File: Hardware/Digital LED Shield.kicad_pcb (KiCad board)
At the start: 2 copper layers, 22 x 26.5 mm, 17 parts, among them IC1 TPS2420RSAT, IC2 LM66200DRLR, J1 Conn_02x10_Odd_Even, J2 Conn_01x03_Male, J3 Barrel_Jack_MountingPin, J4 Conn_01x02_Female, J5 Conn_01x03_Male, U1 SN74LVC1T45DBV

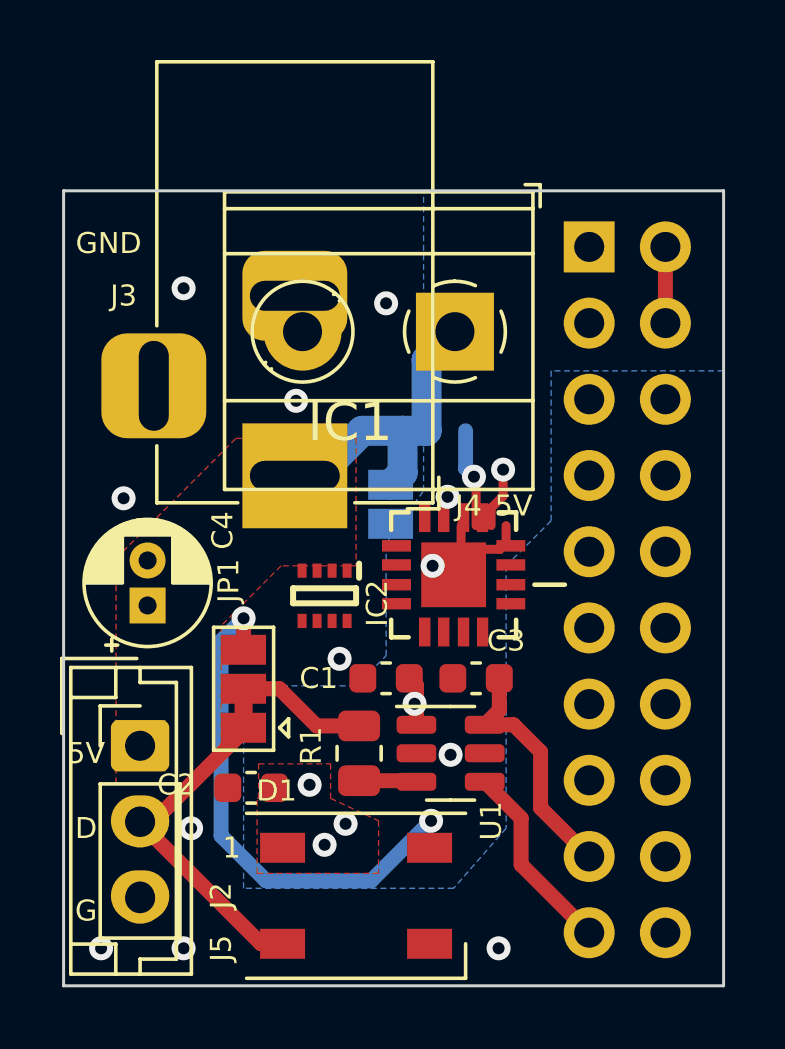
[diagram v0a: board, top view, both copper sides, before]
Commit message: update sch and pcb
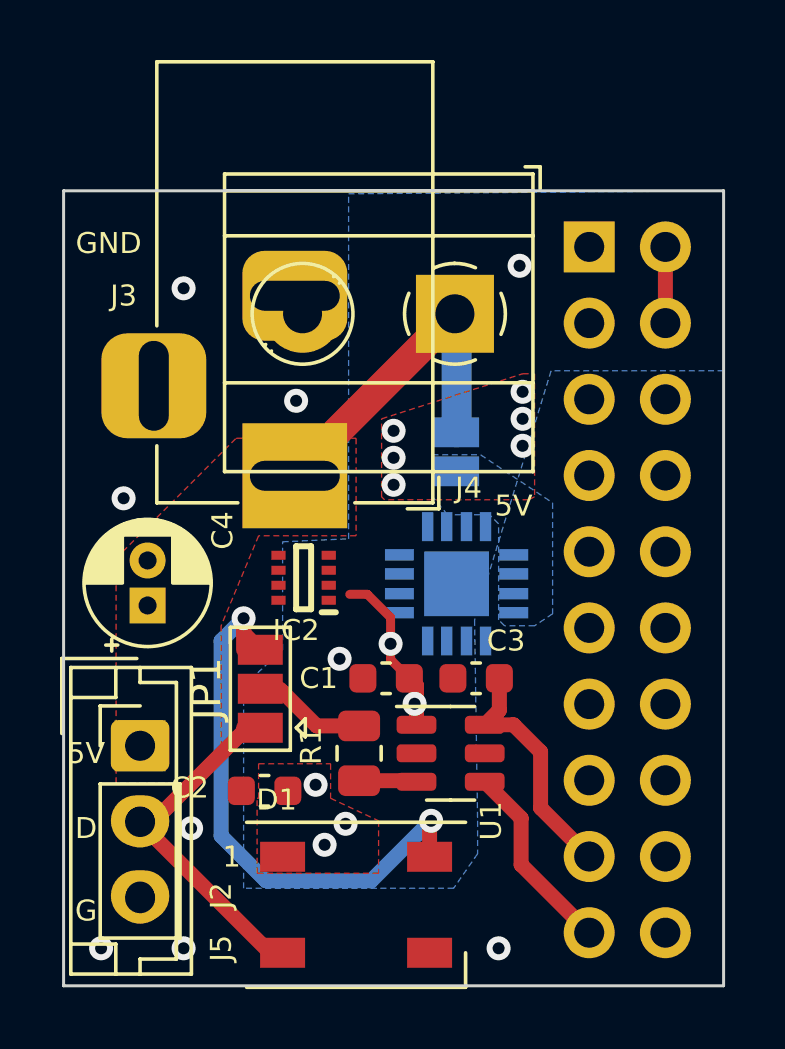
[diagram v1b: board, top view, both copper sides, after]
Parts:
- IC1: moved to B.Cu
- JP1: value Jumper_3_Bridged12 -> Jumper_3_Open; footprint Jumper:SolderJumper-3_P1.3mm_Bridged12_Pad1.0x1.5mm -> Jumper:SolderJumper-3_P1.3mm_Open_Pad1.0x1.5mm
- moved JP2 2.81 mm to (137.1, 92.2)
- moved IC2 0.92 mm to (132.0, 96.4), turned to 180 degrees
- moved J4 0.59 mm to (137.0, 87.6)
- moved JP1 0.56 mm to (130.6, 100.1)
- moved C2 0.46 mm to (130.7, 103.5)
- moved IC1 0.32 mm to (137.1, 96.6), turned to 180 degrees
- moved D1 0.30 mm to (133.8, 107.3)
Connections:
- IC2 pad 2: +5VL -> +5VP
- IC2 pad 3: +5VD -> +5VL
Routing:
- net unconnected-(IC1-Pad13): track 5.34 -> 0.00 mm, vias 1 -> 0
- net +5VP: track 4.19 -> 8.15 mm, vias 6 -> 11
- net GND: track 3.85 -> 0.00 mm, vias 11 -> 9
- net DIN: track 17.1 -> 19.6 mm
- net DOUT: track 10.8 -> 11.6 mm
- net +5V: track 11.0 -> 11.6 mm
- added copper zone on B.Cu, net +5VD
